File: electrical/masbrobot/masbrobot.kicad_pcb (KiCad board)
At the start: 2 copper layers, 61.6 x 40.6 mm, 21 parts, among them J1 TYPE-C-31-M-12, J2 Conn_01x08_MountingPin, Q1 S8050, Q2 S8050, SW1 reset, SW2 boot, U1 CH340G, U2 MPU-6050, U3 ESP32-WROOM-32D, U4 AMS1117-3.3

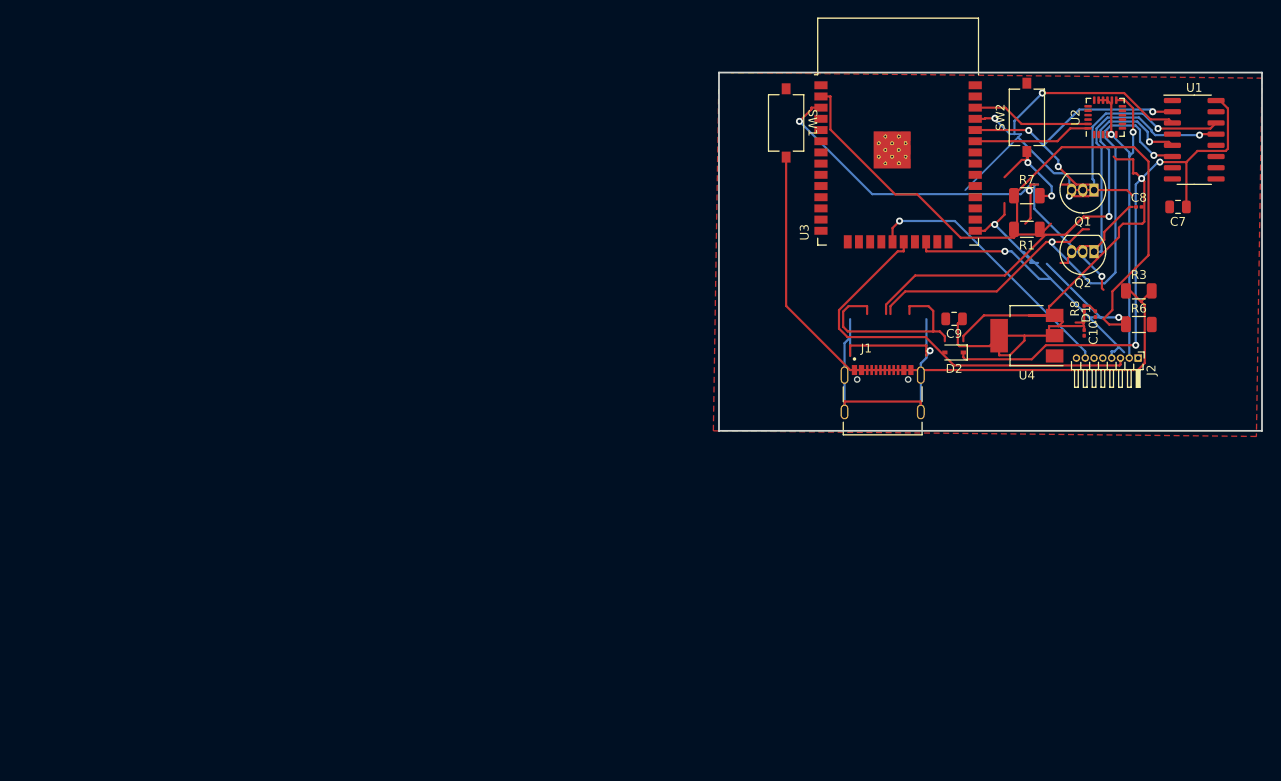
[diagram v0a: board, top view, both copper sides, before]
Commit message: update electrial FIX.
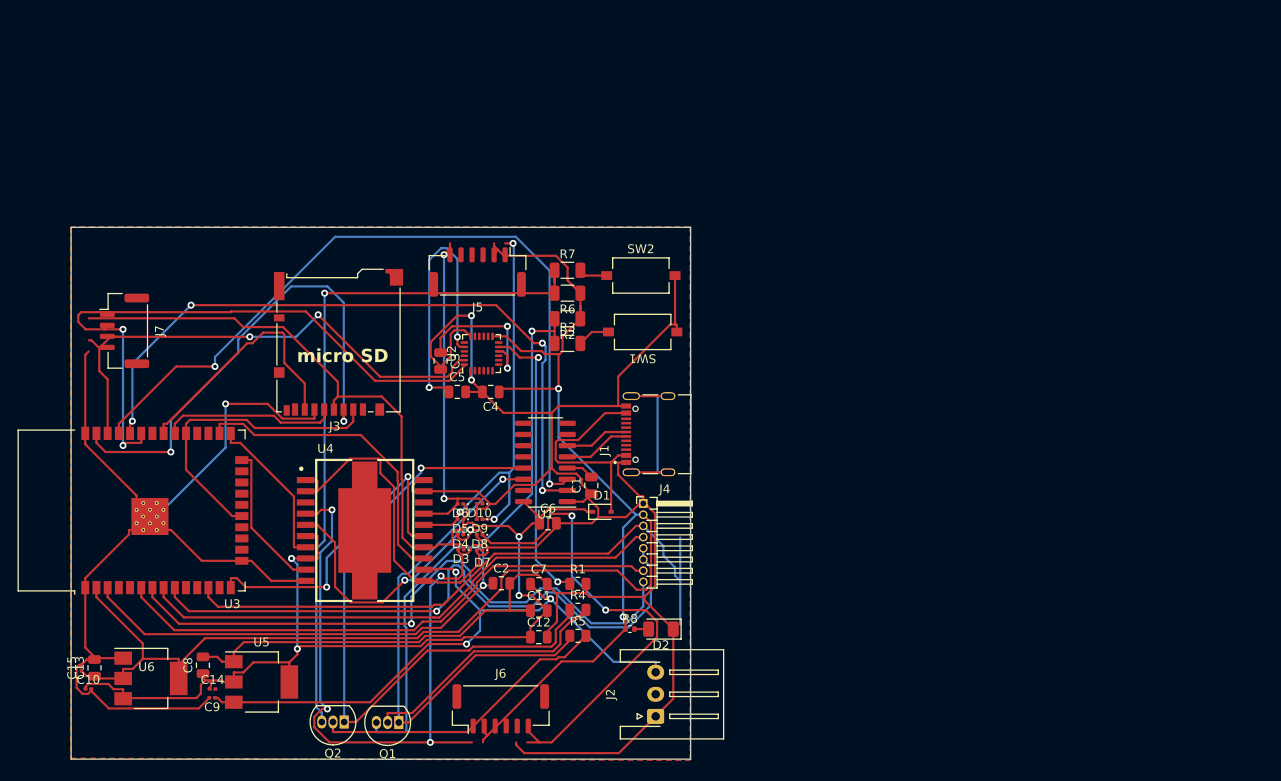
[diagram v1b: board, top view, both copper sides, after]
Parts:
- added C1: 100nF, Capacitor_SMD:C_0805_2012Metric, F.Cu at (130.3, 100.8)
- added C11: 100nF, Capacitor_SMD:C_0805_2012Metric, F.Cu at (124.3, 115.0)
- added C12: 100nF, Capacitor_SMD:C_0805_2012Metric, F.Cu at (124.3, 118.0)
- added C14: 10uF, Capacitor_SMD:C_0201_0603Metric, F.Cu at (87.3, 123.9)
- added C2: 100nF, Capacitor_SMD:C_0805_2012Metric, F.Cu at (120.1, 111.9)
- added C3: 100nF, Capacitor_SMD:C_0805_2012Metric, F.Cu at (113.2, 86.7)
- added C4: 100nF, Capacitor_SMD:C_0805_2012Metric, F.Cu at (118.9, 90.2)
- added C5: 2200pF, Capacitor_SMD:C_0805_2012Metric, F.Cu at (115.1, 90.2)
- added C6: 100nF, Capacitor_SMD:C_0805_2012Metric, F.Cu at (125.4, 105.1)
- added C7: 100nF, Capacitor_SMD:C_0805_2012Metric, F.Cu at (124.3, 112.0)
- added C9: 10uF, Capacitor_SMD:C_0201_0603Metric, F.Cu at (87.3, 124.9)
- added D10: 1N4007, Diode_SMD:D_0201_0603Metric, F.Cu at (117.6, 102.9)
- added D3: 1N4007, Diode_SMD:D_0201_0603Metric, F.Cu at (115.5, 108.1)
- added D4: 1N4007, Diode_SMD:D_0201_0603Metric, F.Cu at (115.5, 106.4)
- added D5: 1N4007, Diode_SMD:D_0201_0603Metric, F.Cu at (115.5, 104.7)
- added D6: 1N4007, Diode_SMD:D_0201_0603Metric, F.Cu at (115.5, 102.9)
- added D7: 1N4007, Diode_SMD:D_0201_0603Metric, F.Cu at (117.6, 108.2)
- added D8: 1N4007, Diode_SMD:D_0201_0603Metric, F.Cu at (117.6, 106.4)
- added D9: 1N4007, Diode_SMD:D_0201_0603Metric, F.Cu at (117.6, 104.7)
- added J2: connector battery 2S Li-Po, Connector_JST:JST_XH_S3B-XH-A-1_1x03_P2.50mm_Horizontal, F.Cu at (137.6, 127.0)
- added J3: Micro_SD_Card, Connector_Card:microSD_HC_Hirose_DM3BT-DSF-PEJS, F.Cu at (101.6, 84.6)
- added J5: Conn_01x06, Connector_JST:JST_GH_BM06B-GHS-TBT_1x06-1MP_P1.25mm_Vertical, F.Cu at (117.4, 76.6)
- added J6: Conn_01x06, Connector_JST:JST_GH_BM06B-GHS-TBT_1x06-1MP_P1.25mm_Vertical, F.Cu at (120.0, 126.2)
- added J7: conn_OLED_128x64_I2C, Connector_JST:JST_GH_BM04B-GHS-TBT_1x04-1MP_P1.25mm_Vertical, F.Cu at (77.3, 83.3)
- added R1: 10k, Resistor_SMD:R_0805_2012Metric, F.Cu at (128.8, 112.0)
- added R4: 10k, Resistor_SMD:R_0805_2012Metric, F.Cu at (128.8, 114.9)
- added R5: 10k, Resistor_SMD:R_0805_2012Metric, F.Cu at (128.8, 117.9)
- added U4: L298P, L298P:SOIC127P1420X360-20N, F.Cu at (104.6, 105.9)
- added U5: AMS1117-5.0, Package_TO_SOT_SMD:SOT-223-3_TabPin2, F.Cu at (92.9, 123.1)
- D2: renamed from D1; footprint LED_SMD:LED_0201_0603Metric -> LED_SMD:LED_1206_3216Metric
- J4: renamed from J2; footprint Connector_PinHeader_1.00mm:PinHeader_1x08_P1.00mm_Horizontal -> Connector_PinHeader_1.27mm:PinHeader_1x08_P1.27mm_Horizontal
- R8: value 1k -> R_LED; footprint Resistor_SMD:R_0201_0603Metric -> Resistor_SMD:R_0402_1005Metric
- moved C10 131.1 mm to (73.2, 123.9)
- moved C8 122.2 mm to (86.2, 121.2), turned to 90 degrees
- moved C15 119.9 mm to (72.5, 121.5), turned to 90 degrees
- moved U6 106.7 mm to (80.3, 122.7), turned to 0 degrees
- moved C13 105.2 mm to (74.0, 121.5), turned to 90 degrees
- moved Q2 100.4 mm to (102.3, 127.6)
- moved Q1 99.3 mm to (108.5, 127.7)
- moved U3 93.0 mm to (81.2, 103.7), turned to 90 degrees
- moved U1 82.2 mm to (125.1, 98.2), turned to 180 degrees
- moved U2 75.6 mm to (117.8, 85.8)
- moved R3 65.1 mm to (127.6, 84.7)
- moved R6 64.9 mm to (127.6, 79.0), turned to 180 degrees
- moved R8 63.1 mm to (134.7, 117.1), turned to 0 degrees
- moved D2 60.9 mm to (138.2, 117.1), turned to 180 degrees
- moved J4 58.5 mm to (136.2, 102.9), turned to 0 degrees
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- renumbered C8 to C10, C9 to C13, C10 to C15, C7 to C8, D2 to D1, R1 to R2, U4 to U6
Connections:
- C13 pad 1: VCC -> +3.3V
- C15 pad 1: VCC -> +3.3V
- J1 pad S1: Net-(J1-SHIELD-PadS1) -> unconnected-(J1-SHIELD-PadS1)
- J1 pad S2: Net-(J1-SHIELD-PadS1) -> unconnected-(J1-SHIELD-PadS1)
- J1 pad S3: Net-(J1-SHIELD-PadS1) -> unconnected-(J1-SHIELD-PadS1)
- J1 pad S4: Net-(J1-SHIELD-PadS1) -> unconnected-(J1-SHIELD-PadS1)
- J4 pad 2: +3V3 -> +3.3V
- J4 pad 3: SCLK -> IO27
- J4 pad 4: DATA -> IO32
- J4 pad 5: RES -> IO33
- J4 pad 6: DC -> IO33
- J4 pad 7: CS -> IO34
- J4 pad 8: BLK -> IO35
- R8 pad 1: VCC -> +3.3V
- U1 pad 7: XI -> unconnected-(U1-XI-Pad7)
- U1 pad 8: XO -> unconnected-(U1-XO-Pad8)
- U2 pad 13: +3V3 -> +3.3V
- U3 pad 14: IO12 -> IN4
- U3 pad 24: IO2 -> IN2
- U3 pad 25: IO0 -> IN1
- U3 pad 26: IO4 -> IN3
- U3 pad 29: IO5 -> CS
- U3 pad 30: IO18 -> SCK
- U3 pad 31: IO19 -> MISO
- U3 pad 37: IO23 -> MOSI
- U6 pad 2: VCC -> +3.3V
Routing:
- net GNDREF: track 0.00 -> 415.4 mm, vias 0 -> 3
- net +3.3V: track 81.3 -> 192.4 mm, vias 0 -> 2
- net M1B: track 0.00 -> 88.3 mm, vias 0 -> 4
- net +5V: track 103.5 -> 183.9 mm, vias 3 -> 4
- net M1A: track 0.00 -> 76.7 mm, vias 0 -> 4
- net +7.5V: track 0.00 -> 72.8 mm, vias 0 -> 3
- net IO33: track 0.00 -> 72.5 mm, vias 0 -> 1
- net IO27: track 0.00 -> 72.5 mm
- net IO35: track 0.00 -> 71.3 mm, vias 0 -> 1
- net Net-(R3-Pad2): track 71.6 -> 3.73 mm
- net IO34: track 0.00 -> 63.0 mm
- net EN: track 55.5 -> 117.8 mm, vias 3 -> 2
- net IO32: track 0.00 -> 60.4 mm
- net SDA: track 13.4 -> 71.3 mm, vias 0 -> 2
- net D-: track 63.8 -> 7.31 mm, vias 2 -> 0
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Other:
- board size 61.6 x 40.6 mm -> 70.3 x 60.3 mm
- board text added: "micro SD"
